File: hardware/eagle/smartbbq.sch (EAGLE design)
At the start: 30 parts, among them X1 KLBR1, X2 KLBR1, X3 KLBR1, X4 KLBR1

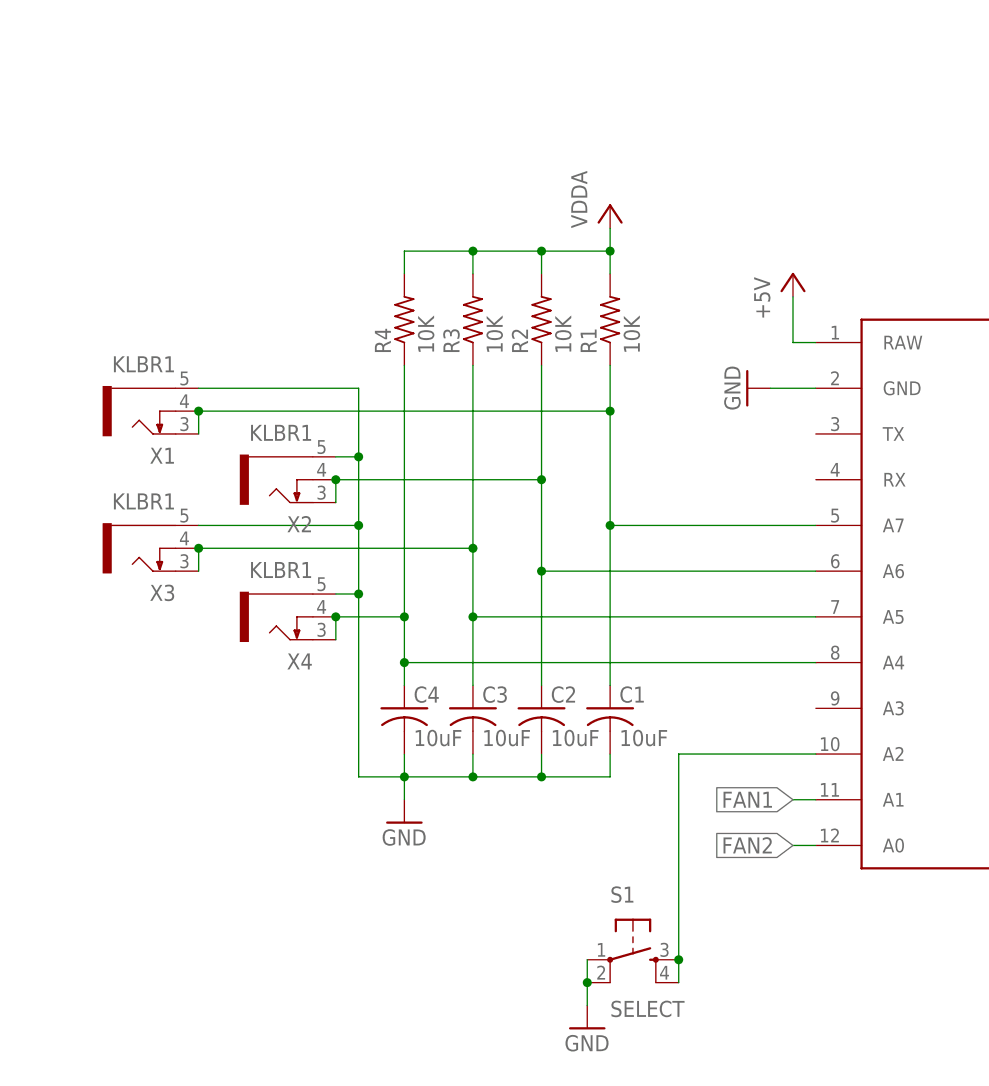
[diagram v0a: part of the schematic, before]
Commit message: Piezo addition
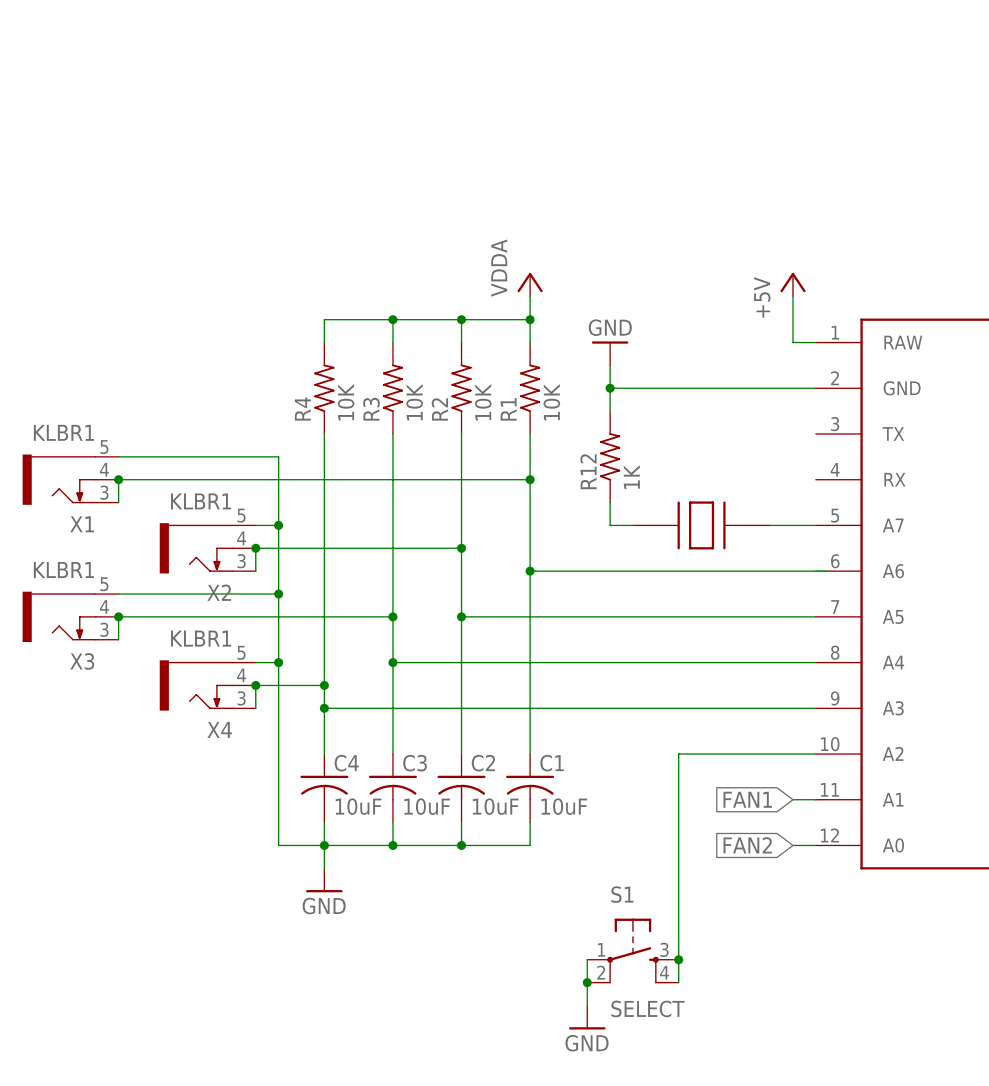
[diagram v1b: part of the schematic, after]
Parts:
- added R12: 1K, rcl:R-US_R0603
- added U$2: CMT_1603_SMT, engirati:CMT_1603_SMT
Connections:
- new net N$28: R12.1, U$2.P$1
- new net N$29: U$1.A7, U$2.P$2
- net GND: now also R12.2
- net N$15: no longer U$1.A7
- net N$17: now also U$1.A5; no longer U$1.A6
- net N$18: now also U$1.A4; no longer U$1.A5
- net N$19: now also U$1.A3; no longer U$1.A4
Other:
- moved on the sheet: C1, C2, C3, C4, R1, R2, R3, R4, X1, X2, X3, X4
